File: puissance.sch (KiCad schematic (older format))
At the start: 28 parts, among them J12 ZMCT103C, J2 Conn_01x04_Male, K2 Finder 40.62.9.024V, K3 Finder 40.61.9.024V, K4 Finder 40.61.9.024V, Q2 BS170, Q3 BS170, Q4 BS170, Q5 BTA26-600-BWRG, U3 MOC3020M

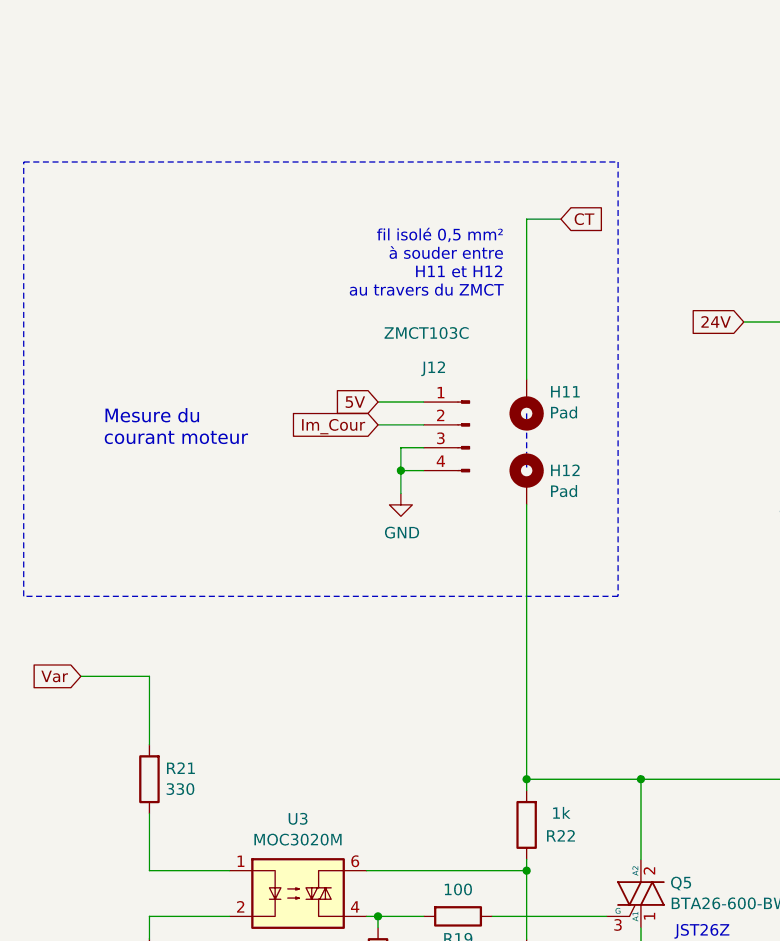
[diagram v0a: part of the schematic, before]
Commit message: V2.32
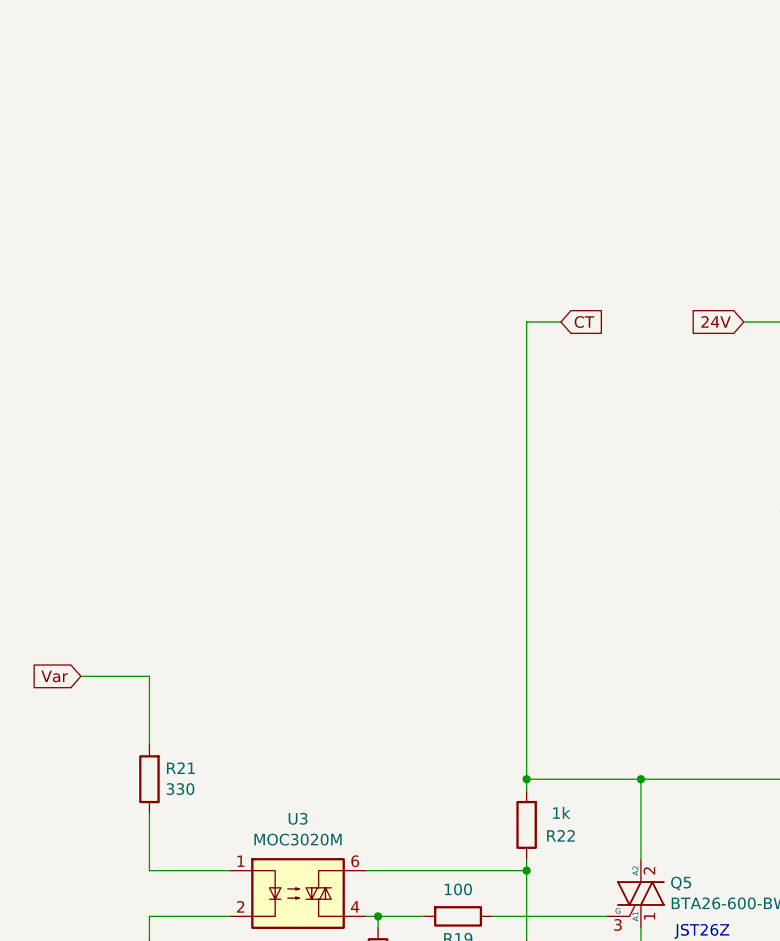
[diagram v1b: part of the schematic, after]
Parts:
- removed H11, H12: Pad, MountingHole:MountingHole_2.2mm_M2_Pad, symbol Mechanical:MountingHole_Pad
- removed J12: ZMCT103C, Connector_PinSocket_2.54mm:PinSocket_1x04_P2.54mm_Vertical, symbol Connector:Conn_01x04_Male
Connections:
- net CT: now also Q5.2 (A2), R22.2, R29.2
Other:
- note removed: "Mesure du \ncourant moteur"
- note removed: "fil isolé 0,5 mm²\nà souder entre\nH11 et H12\nau travers du ZMCT"
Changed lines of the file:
@@
 	4150 3150 4600 3150
 Connection ~ 4600 3150
-Text Notes 3100 3050 2    50   ~ 0
-fil isolé 0,5 mm²\nà souder entre\nH11 et H12\nau travers du ZMCT
 Wire Wire Line
 	7100 3150 8750 3150
@@
 Connection ~ 3200 5550
 Wire Wire Line
-	3200 5550 3200 5850
-Wire Wire Line
 	2500 5550 3200 5550
 Wire Wire Line
@@
 	4600 5500 4600 5850
 Connection ~ 3200 5150
-Wire Wire Line
-	3200 3950 3200 5150
-Text GLabel 3350 2700 2    50   Input ~ 0
+Text GLabel 3350 3150 2    50   Input ~ 0
 CT
-$Comp
-L Mechanical:MountingHole_Pad H11
-U 1 1 6122C890
-P 3200 3500
-F 0 "H11" H 3100 3457 50  0000 R CNN
-F 1 "Pad" H 3100 3548 50  0000 R CNN
-F 2 "MountingHole:MountingHole_2.2mm_M2_Pad" H 3200 3500 50  0001 C CNN
-F 3 "~" H 3200 3500 50  0001 C CNN
-	1    3200 3500
-	-1   0    0    1
-$EndComp
-$Comp
-L Mechanical:MountingHole_Pad H12
-U 1 1 6122B8CD
-P 3200 3850
-F 0 "H12" H 3300 3899 50  0000 L CNN
-F 1 "Pad" H 3300 3808 50  0000 L CNN
-F 2 "MountingHole:MountingHole_2.2mm_M2_Pad" H 3200 3850 50  0001 C CNN
-F 3 "~" H 3200 3850 50  0001 C CNN
-	1    3200 3850
-	1    0    0    -1
-$EndComp
-Wire Wire Line
-	3200 2700 3200 3400
 $Comp
 L power:GND #PWR?
@@
 Wire Wire Line
 	4650 4700 4650 4800
-Wire Notes Line
-	3200 3550 3200 3800
-Wire Notes Line
-	3600 4350 1000 4350
-Wire Notes Line
-	1000 2450 3600 2450
-Text GLabel 2550 3600 0    50   Input ~ 0
-Im_Cour
 Wire Wire Line
-	3200 2700 3350 2700
-Text Notes 1350 3700 0    59   ~ 0
-  Mesure du \ncourant moteur
-$Comp
-L Connector:Conn_01x04_Male J?
-U 1 1 61368E20
-P 2950 3600
-AR Path="/61368E20" Ref="J?"  Part="1"
-AR Path="/6130ED2A/61368E20" Ref="J12"  Part="1"
-F 0 "J12" H 3050 3850 50  0000 L CNN
-F 1 "ZMCT103C" H 2950 4000 50  0000 L CNN
-F 2 "Connector_PinSocket_2.54mm:PinSocket_1x04_P2.54mm_Vertical" H 2950 3600 50  0001 C CNN
-F 3 "~" H 2950 3600 50  0001 C CNN
-	1    2950 3600
-	-1   0    0    -1
-$EndComp
-$Comp
-L power:GND #PWR?
-U 1 1 6136AA8A
-P 2650 3900
-AR Path="/6136AA8A" Ref="#PWR?"  Part="1"
-AR Path="/6130ED2A/6136AA8A" Ref="#PWR021"  Part="1"
-F 0 "#PWR021" H 2650 3650 50  0001 C CNN
-F 1 "GND" H 2655 3727 50  0000 C CNN
-F 2 "" H 2650 3900 50  0001 C CNN
-F 3 "" H 2650 3900 50  0001 C CNN
-	1    2650 3900
-	1    0    0    -1
-$EndComp
+	3200 3150 3350 3150
 Wire Wire Line
-	2750 3700 2650 3700
+	3200 3150 3200 5150
 Wire Wire Line
-	2650 3700 2650 3800
-Wire Wire Line
-	2750 3800 2650 3800
-Connection ~ 2650 3800
-Wire Wire Line
-	2650 3800 2650 3900
-Wire Wire Line
-	2550 3600 2750 3600
-Wire Wire Line
-	2750 3500 2550 3500
-Text GLabel 2550 3500 0    50   Input ~ 0
-5V
-Wire Notes Line
-	1000 4350 1000 2450
-Wire Notes Line
-	3600 2450 3600 4350
+	3200 5550 3200 5850
 $EndSCHEMATC
